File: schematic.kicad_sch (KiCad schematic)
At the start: 5 parts, among them J1 AudioJack3_SwitchT, J2 Barrel_Jack_Switch, J3 Screw_Terminal_01x02, J4 Screw_Terminal_01x02, U1 PAM8610

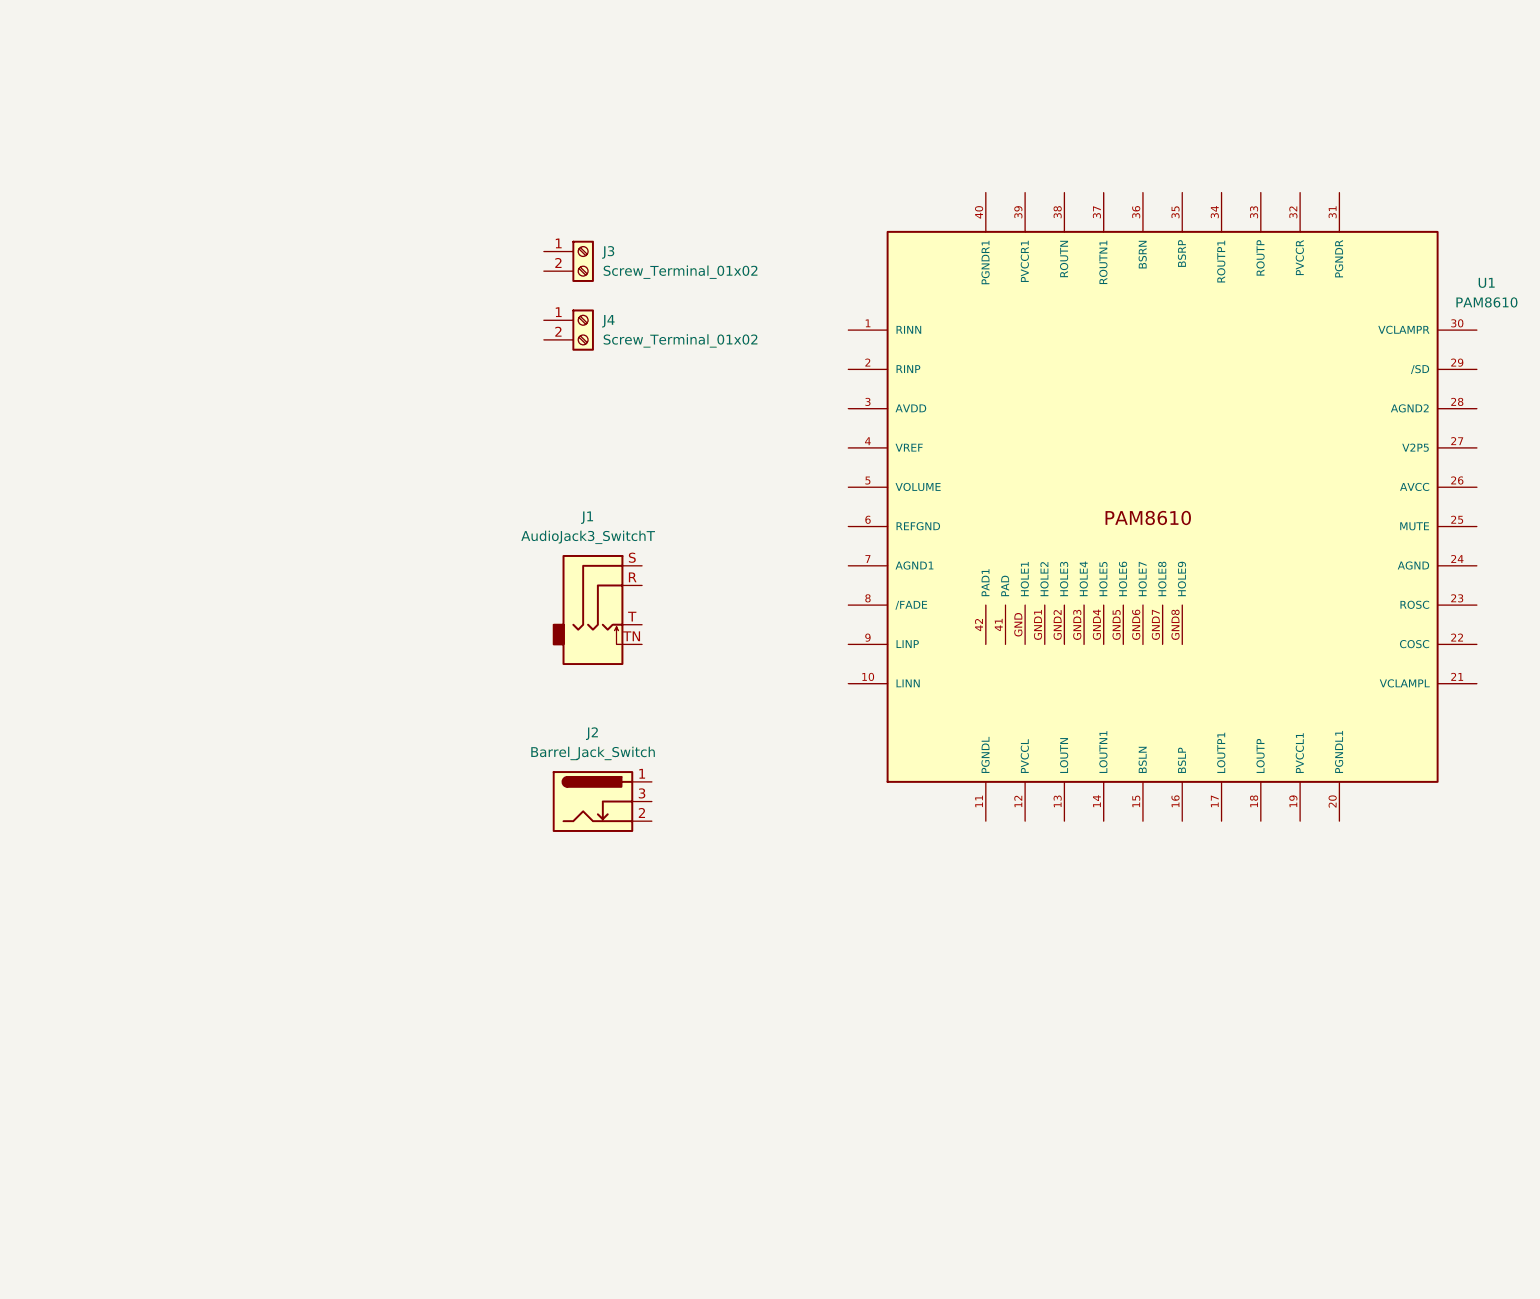
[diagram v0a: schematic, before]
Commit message: Add files via upload
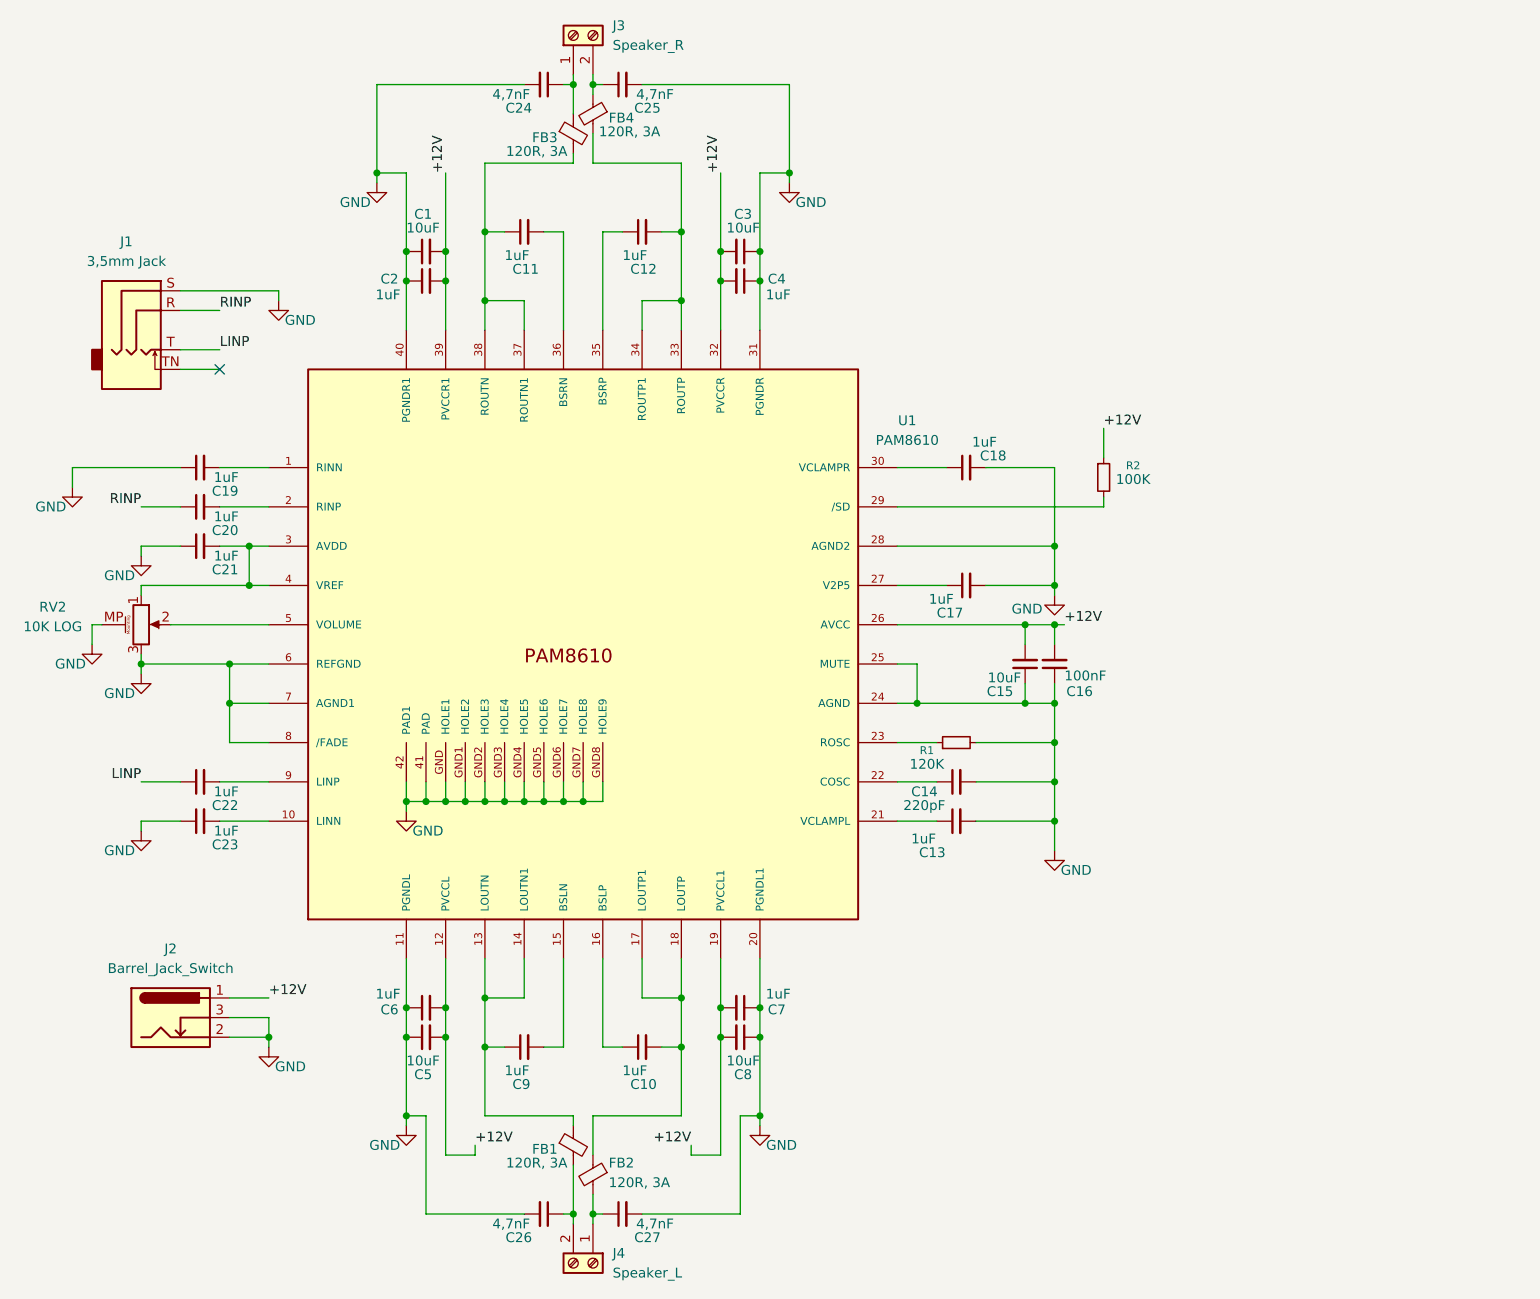
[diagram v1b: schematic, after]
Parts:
- added C1, C15, C3, C5, C8: 10uF, symbol Device:C_Small
- added C10, C11, C12, C13, C17, C18, C19, C2, C20, C21, C22, C23, C4, C6, C7, C9: 1uF, symbol Device:C_Small
- added C14: 220pF, symbol Device:C_Small
- added C16: 100nF, symbol Device:C_Small
- added C24, C25, C26, C27: 4,7nF, symbol Device:C_Small
- added FB1, FB2, FB3, FB4: 120R, 3A, symbol Device:FerriteBead_Small
- added R1: 120K, symbol Device:R_Small
- added R2: 100K, symbol Device:R_Small
- added RV2: 10K LOG, Potentiometer_THT:AudioPot, symbol Device:R_Potentiometer_MountingPin
- J1: value AudioJack3_SwitchT -> 3,5mm Jack
- J3: value Screw_Terminal_01x02 -> Speaker_R
- J4: value Screw_Terminal_01x02 -> Speaker_L
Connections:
- net +12V: now reaches J2.1
- net +12V: now also U1.12 (PVCCL), U1.19 (PVCCL1), U1.26 (AVCC), U1.32 (PVCCR), U1.39 (PVCCR1), C1.2, C15.2, C16.2, C2.2, C3.2, C4.2, C5.2, C6.2, C7.2, C8.2, R2.1
- net GND: now reaches J2.2
- net GND: now also J1.S, J2.3, U1.11 (PGNDL), U1.20 (PGNDL1), U1.24 (AGND), U1.25 (MUTE), U1.28 (AGND2), U1.31 (PGNDR), U1.40 (PGNDR1), U1.41 (PAD), U1.42 (PAD1), U1.6 (REFGND), U1.7 (AGND1), U1.8 (/FADE), U1.GND (HOLE1), U1.GND1 (HOLE2), U1.GND2 (HOLE3), U1.GND3 (HOLE4), U1.GND4 (HOLE5), U1.GND5 (HOLE6), U1.GND6 (HOLE7), U1.GND7 (HOLE8), U1.GND8 (HOLE9), C1.1, C13.2, C14.2, C15.1, C16.1, C17.2, C18.2, C19.1, C2.1, C21.1, C23.1, C24.2, C25.2, C26.2, C27.2, C3.1, C4.1, C5.1, C6.1, C7.1, C8.1, R1.2, RV2.3, RV2.MP (MountPin)
- net RINP: now reaches J1.R
- net RINP: now also C20.1
- net LINP: now reaches J1.T
- net LINP: now also C22.1
- net at J4.1 (Pin_1): now also C27.1, FB2.2
- net at J4.2 (Pin_2): now also C26.1, FB1.2
- net at U1.1 (RINN): now also C19.2
- net at U1.10 (LINN): now also C23.2
- net at U1.13 (LOUTN): now also U1.14 (LOUTN1), C9.1, FB1.1
- net at U1.15 (BSLN): now also C9.2
- net at U1.16 (BSLP): now also C10.1
- net at U1.17 (LOUTP1): now also U1.18 (LOUTP), C10.2, FB2.1
- net at U1.2 (RINP): now also C20.2
- net at U1.21 (VCLAMPL): now also C13.1
- net at U1.22 (COSC): now also C14.1
- net at U1.23 (ROSC): now also R1.1
- net at U1.27 (V2P5): now also C17.1
- net at U1.29 (/SD): now also R2.2
- net at U1.3 (AVDD): now also U1.4 (VREF), C21.2, RV2.1
- net at U1.30 (VCLAMPR): now also C18.1
- net at U1.33 (ROUTP): now also U1.34 (ROUTP1), C12.2, FB4.2
- net at U1.35 (BSRP): now also C12.1
- net at U1.36 (BSRN): now also C11.2
- net at U1.37 (ROUTN1): now also U1.38 (ROUTN), C11.1, FB3.2
- net at U1.5 (VOLUME): now also RV2.2
- net at U1.9 (LINP): now also C22.2
- net at J3.1 (Pin_1): now also C24.1, FB3.1
- net at J3.2 (Pin_2): now also C25.1, FB4.1
- no-connect marks 0 -> 1
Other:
- moved on the sheet: J1, J2, J3, J4, U1
